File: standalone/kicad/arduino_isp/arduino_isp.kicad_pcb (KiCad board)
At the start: 2 copper layers, 70.5 x 50 mm, 9 parts, among them J1 ICSP, J2 Conn_01x10, J3 Conn_01x06

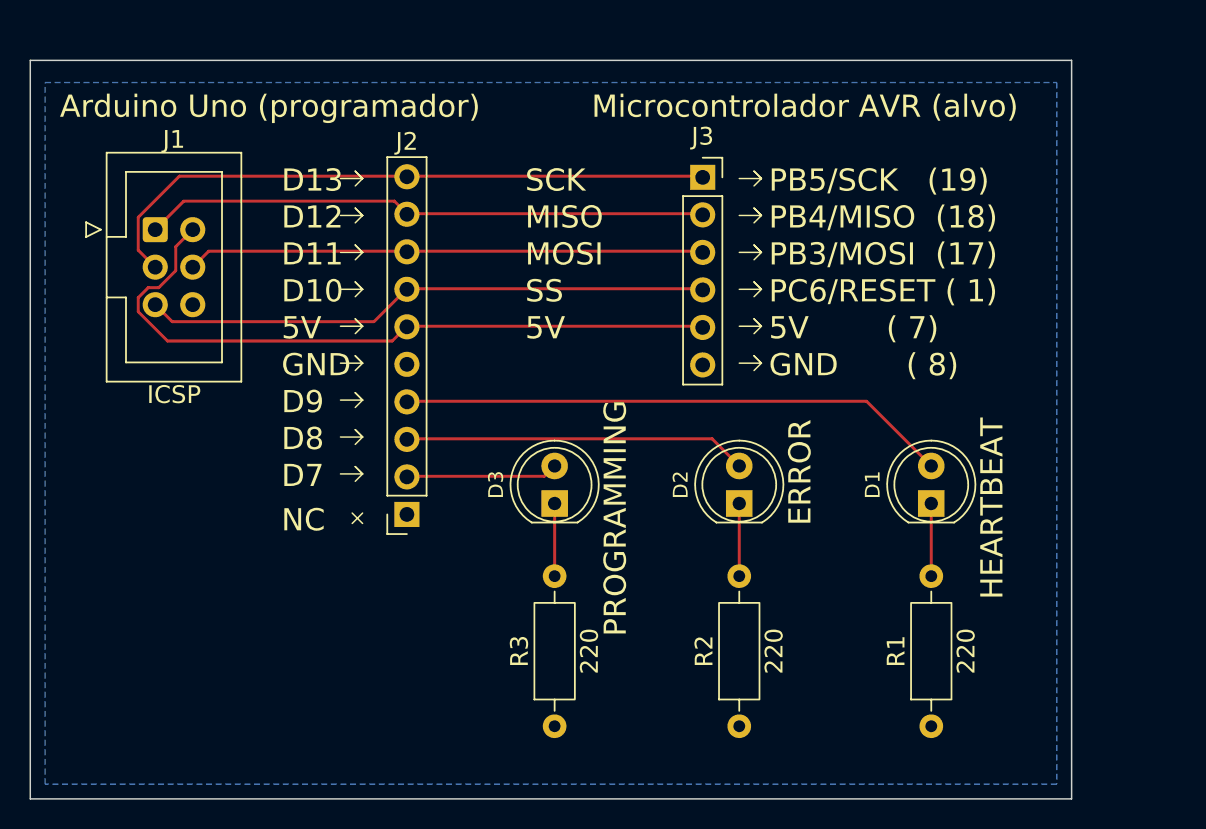
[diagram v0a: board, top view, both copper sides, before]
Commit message: Finalização da placa Aruino ISP
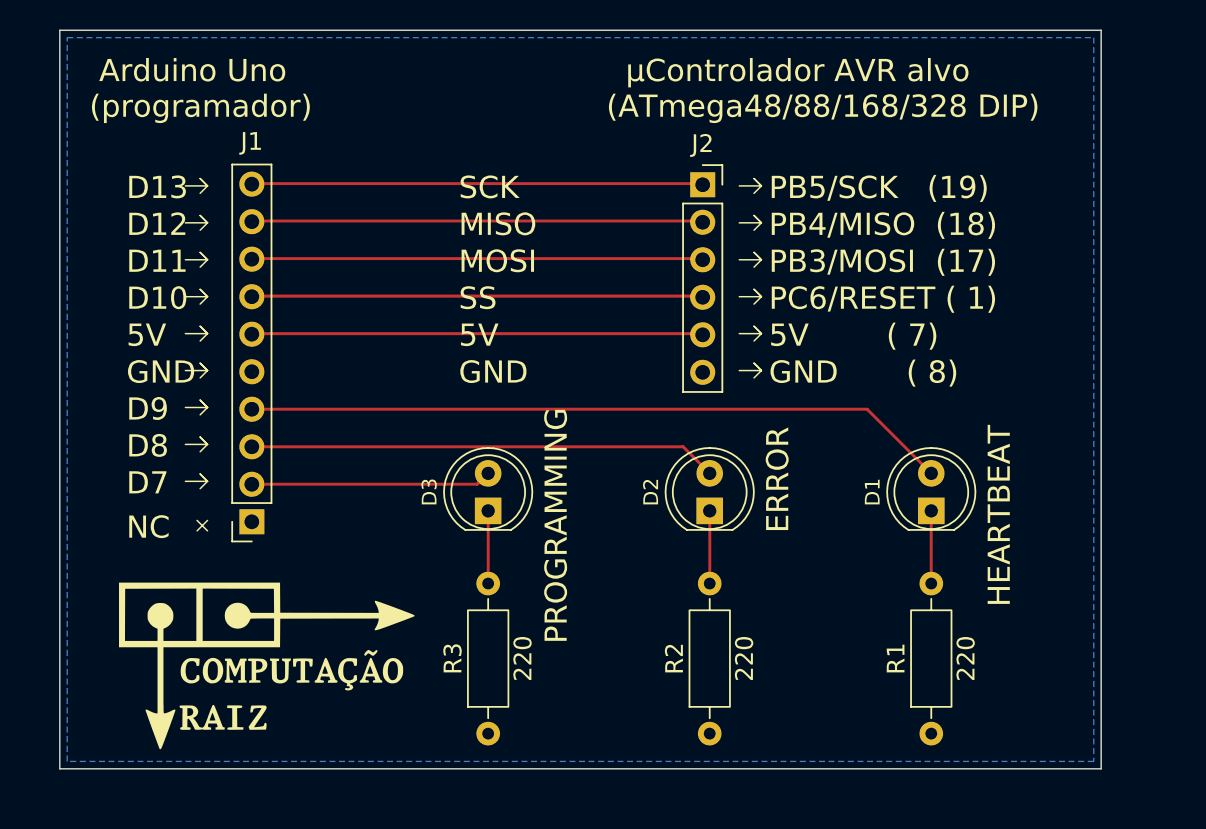
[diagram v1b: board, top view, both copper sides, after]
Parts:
- removed the J1 at (90.5, 50.5)
- added G***: LOGO, logo_computacao_raiz:logo_computacao_raiz_20x11mm, F.Cu at (98.0, 80.0)
- moved J1 10.5 mm to (97.0, 70.2)
- moved D3 4.53 mm to (113.0, 69.5)
- moved R3 4.53 mm to (113.0, 84.6)
- moved D2 2.06 mm to (128.0, 69.5)
- moved R2 2.06 mm to (128.0, 84.6)
- moved D1 0.50 mm to (143.0, 69.5)
- moved J2 0.50 mm to (127.5, 47.4)
- moved R1 0.50 mm to (143.0, 84.6)
- renumbered J2 to J1, J3 to J2
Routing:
- net +5V: track 47.0 -> 30.6 mm
- net /SCK: track 43.3 -> 30.6 mm
- net Net-(D1-A): track 37.3 -> 47.8 mm
- net Net-(D2-A): track 23.3 -> 31.7 mm
- net /SS: track 38.5 -> 30.6 mm
- net /MISO: track 38.7 -> 31.0 mm
- net Net-(D3-A): track 10.3 -> 16.3 mm
- net /MOSI: track 35.0 -> 30.6 mm
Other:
- board text added: "μControlador AVR alvo (ATmega48/88/168/328 DIP)"
- board text removed: "Microcontrolador AVR (alvo)"
